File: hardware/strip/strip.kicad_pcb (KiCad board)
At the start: 4 copper layers, 66 x 18 mm, 40 parts, among them J101 Cortex, J102 DX07S016JA3, J201 WAGO 2065-100, J202 WAGO 2065-100, J203 WAGO 2065-100, SW101 SKSG, SW102 SKSG, U101 ATSAMD51G, U102 TPS78433QWDRBRQ1, U201 74AHC1G125, Y101 32k768

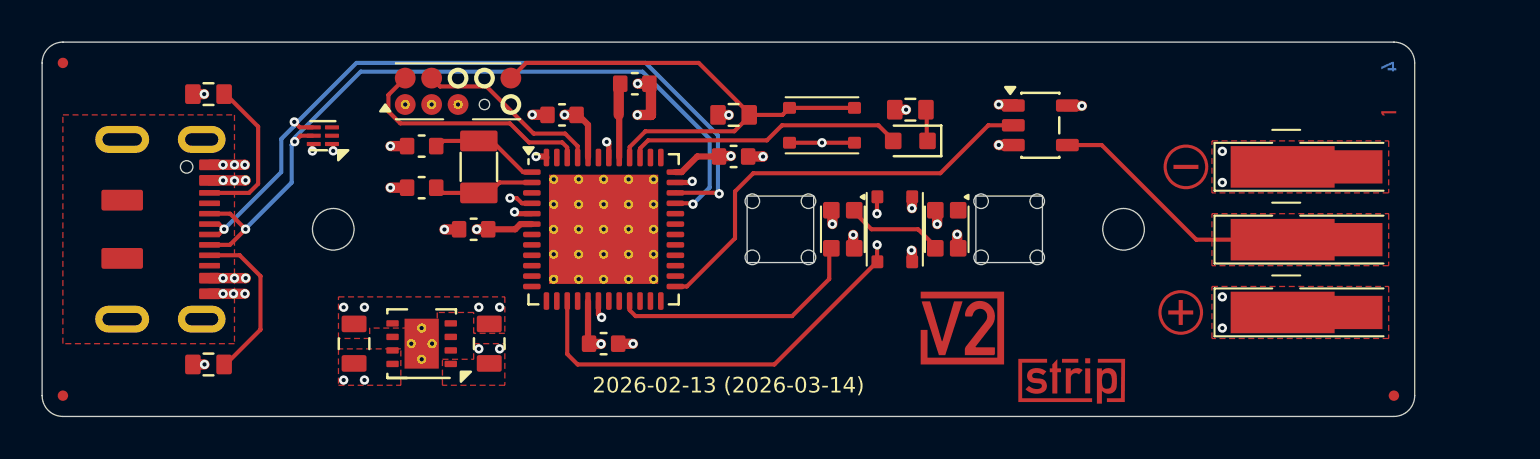
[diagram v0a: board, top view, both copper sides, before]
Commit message: Update
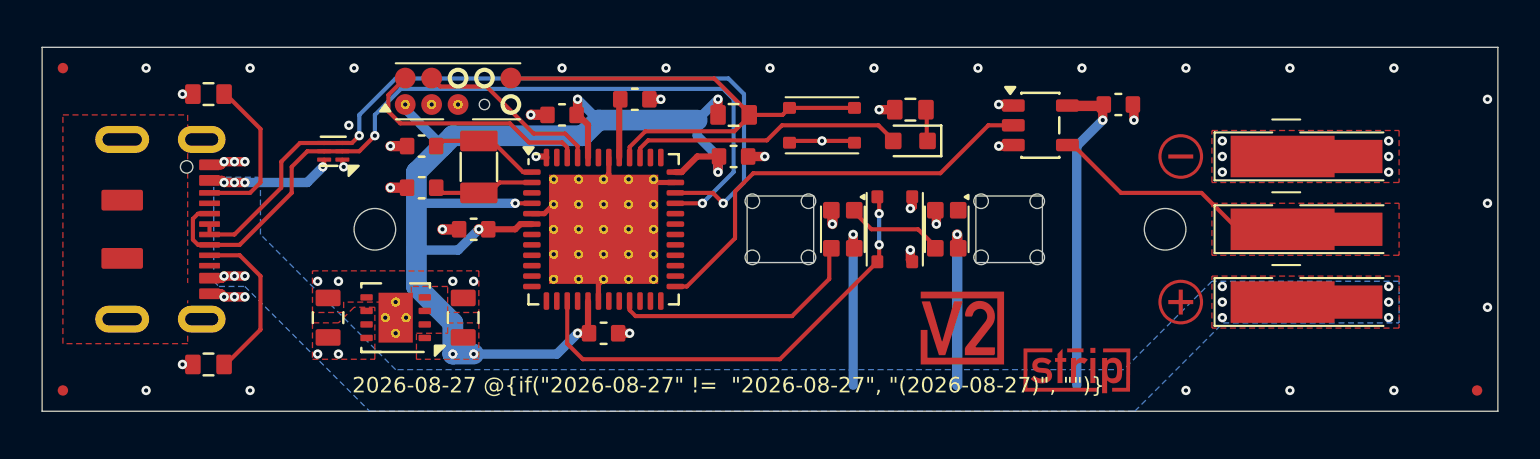
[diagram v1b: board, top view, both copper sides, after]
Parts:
- added C201: 0u1, V2_Capacitor_SMD:C_1608, F.Cu at (168.8, 100.0)
- C101, C102, C103, C104, C105, C106, C107: footprint V2_Capacitor_SMD:C_0603 -> V2_Capacitor_SMD:C_1608
- C108, C109: footprint V2_Capacitor_SMD:C_0805 -> V2_Capacitor_SMD:C_2012
- D101: footprint V2_LED:LED_0603 -> V2_LED:LED_1608
- INFO102: value Layer_Numbers -> Layer_Numbers-4; footprint V2_Production:Layer_Numbers -> V2_Production:Layer_Numbers-4
- R101, R102, R103, R104: footprint V2_Resistor_SMD:R_0603 -> V2_Resistor_SMD:R_1608
- moved INFO102 14.7 mm to (179.5, 113.8), turned to 0 degrees
- moved FID103 4.01 mm to (186.0, 113.8)
- moved H101 2.00 mm to (133.0, 106.0)
- moved H102 2.00 mm to (171.0, 106.0)
- moved C108 1.77 mm to (130.8, 110.2)
- moved C109 1.77 mm to (137.2, 110.2)
- moved U102 1.77 mm to (134.0, 110.2)
- moved ESD101 0.90 mm to (131.0, 102.2)
- moved C103 0.75 mm to (145.5, 99.8)
- moved ICON101 0.56 mm to (166.8, 112.8)
- moved ICON103 0.56 mm to (171.8, 102.5)
- moved C106 0.50 mm to (144.0, 111.0)
- moved ICON104 0.50 mm to (171.8, 109.5)
- moved J201 0.50 mm to (177.2, 109.5)
- moved J202 0.50 mm to (177.2, 102.5)
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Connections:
- ESD101 pad 2: unconnected-(ESD101-D2-Pad2) -> /USB-
- ESD101 pad 3: unconnected-(ESD101-D1-Pad3) -> /USB+
- U102 pad 6: unconnected-(U102-Pad6) -> +5V
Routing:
- net +3V3: track 13.1 -> 59.5 mm
- net +5V: track 6.03 -> 39.9 mm, vias 14 -> 18
- net /USB-: track 37.4 -> 39.6 mm, vias 3 -> 2
- net /USB+: track 37.1 -> 39.1 mm, vias 3 -> 2
- net /VDDCORE: track 3.56 -> 2.82 mm
- net /RESET: track 25.0 -> 24.4 mm
- net GND: track 23.8 -> 23.6 mm, vias 36 -> 57
- added copper zone on B.Cu, net +5V
- removed copper zone on In2.Cu, net +3V3
- removed copper zone on In2.Cu, net +5V
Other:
- board size 66 x 18 mm -> 70 x 17.5 mm
